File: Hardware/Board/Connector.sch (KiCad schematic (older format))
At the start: 7 parts, among them J10 WAGO_Klemmleiste_8-pol, J11 RJ12, J12 RJ45, J13 WAGO_Klemmleiste_6-pol, J7 WAGO_Klemmleiste_6-pol, J8 WAGO_Klemmleiste_4-pol, J9 WAGO_Klemmleiste_8-pol

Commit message: Eine Menge Arbeit auf der GPN, fast fertig im Schaltplan.
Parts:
- J10, J9: symbol WAGO~Klemmleisten:WAGO_Klemmleiste_8-pol -> Womo-rescue:WAGO_Klemmleiste_8-pol-WAGO_Klemmleisten
- J13, J7: symbol WAGO~Klemmleisten:WAGO_Klemmleiste_6-pol -> Womo-rescue:WAGO_Klemmleiste_6-pol-WAGO_Klemmleisten
- J8: symbol WAGO~Klemmleisten:WAGO_Klemmleiste_4-pol -> Womo-rescue:WAGO_Klemmleiste_4-pol-WAGO_Klemmleisten
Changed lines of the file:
@@
 EESchema Schematic File Version 4
 LIBS:Womo-cache
-EELAYER 26 0
+EELAYER 29 0
 EELAYER END
 $Descr A4 11693 8268
 encoding utf-8
-Sheet 7 7
+Sheet 6 7
 Title ""
 Date ""
@@
 $EndDescr
 $Comp
-L WAGO~Klemmleisten:WAGO_Klemmleiste_4-pol J8
+L Womo-rescue:WAGO_Klemmleiste_4-pol-WAGO_Klemmleisten J8
 U 1 1 5CB5F9FC
 P 1900 950
@@
 $EndComp
 $Comp
-L WAGO~Klemmleisten:WAGO_Klemmleiste_8-pol J9
+L Womo-rescue:WAGO_Klemmleiste_8-pol-WAGO_Klemmleisten J9
 U 1 1 5CB5FBA8
 P 1900 2050
@@
 $EndComp
 $Comp
-L WAGO~Klemmleisten:WAGO_Klemmleiste_8-pol J10
+L Womo-rescue:WAGO_Klemmleiste_8-pol-WAGO_Klemmleisten J10
 U 1 1 5CB5FC2E
 P 1900 3450
@@
 $EndComp
 $Comp
-L WAGO~Klemmleisten:WAGO_Klemmleiste_6-pol J7
+L Womo-rescue:WAGO_Klemmleiste_6-pol-WAGO_Klemmleisten J7
 U 1 1 5CBD1756
 P 1850 5700
@@
 	700  600  700  1450
 $Comp
-L WAGO~Klemmleisten:WAGO_Klemmleiste_6-pol J13
+L Womo-rescue:WAGO_Klemmleiste_6-pol-WAGO_Klemmleisten J13
 U 1 1 5CBE3A31
 P 5250 1050

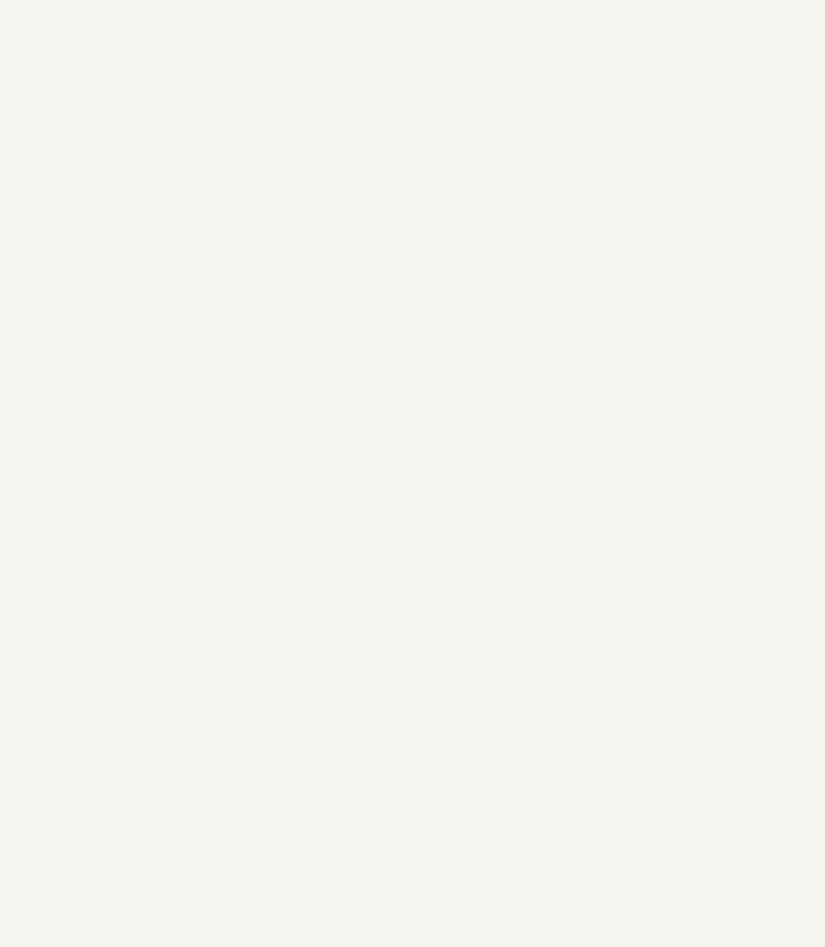
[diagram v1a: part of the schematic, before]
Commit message: Board to Board Verbindung eingefügt
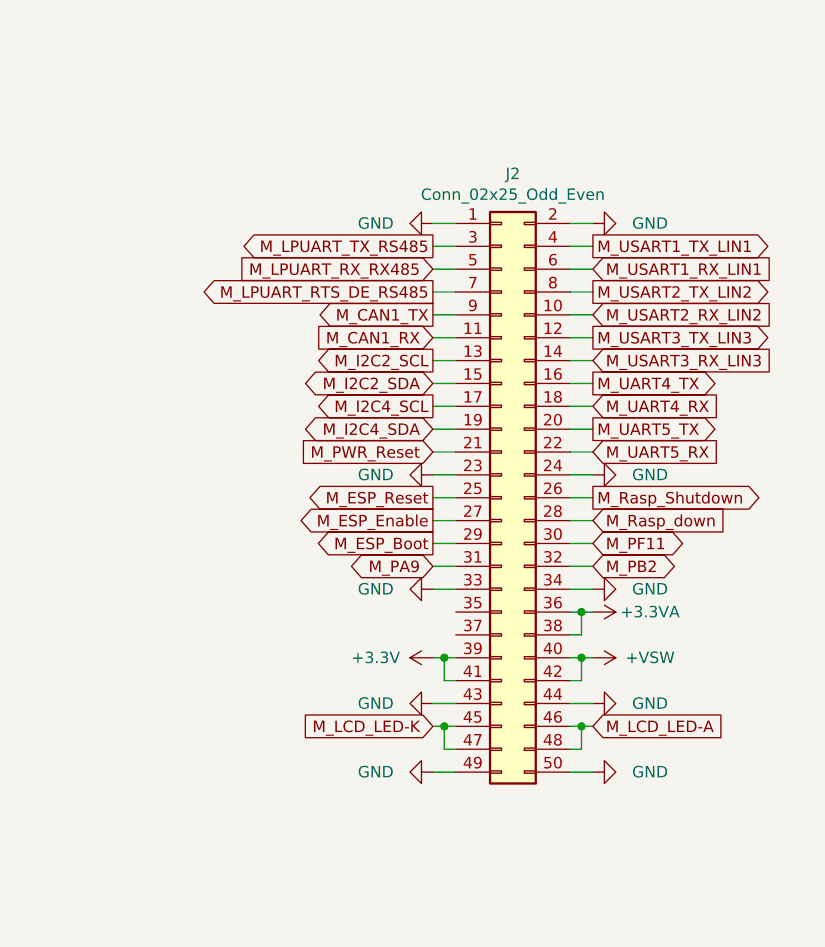
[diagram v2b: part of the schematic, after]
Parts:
- added J2: Conn_02x25_Odd_Even, Connector_PinSocket_2.54mm:PinSocket_2x25_P2.54mm_Vertical, symbol Connector_Generic:Conn_02x25_Odd_Even
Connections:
- net GND: now also J2.1 (Pin_1), J2.2 (Pin_2), J2.23 (Pin_23), J2.24 (Pin_24), J2.33 (Pin_33), J2.34 (Pin_34), J2.43 (Pin_43), J2.44 (Pin_44), J2.49 (Pin_49), J2.50 (Pin_50)
- new net +3.3VA: J2.36 (Pin_36), J2.38 (Pin_38)
- new net +3V3: J2.39 (Pin_39), J2.41 (Pin_41)
- new net +VSW: J2.40 (Pin_40), J2.42 (Pin_42)
- new net M_CAN1_RX: J2.11 (Pin_11)
- new net M_CAN1_TX: J2.9 (Pin_9)
- new net M_ESP_Boot: J2.29 (Pin_29)
- new net M_ESP_Enable: J2.27 (Pin_27)
- new net M_ESP_Reset: J2.25 (Pin_25)
- new net M_I2C2_SCL: J2.13 (Pin_13)
- new net M_I2C2_SDA: J2.15 (Pin_15)
- new net M_I2C4_SCL: J2.17 (Pin_17)
- new net M_I2C4_SDA: J2.19 (Pin_19)
- new net M_LCD_LED-A: J2.46 (Pin_46), J2.48 (Pin_48)
- new net M_LCD_LED-K: J2.45 (Pin_45), J2.47 (Pin_47)
- new net M_LPUART_RTS_DE_RS485: J2.7 (Pin_7)
- new net M_LPUART_RX_RX485: J2.5 (Pin_5)
- new net M_LPUART_TX_RS485: J2.3 (Pin_3)
- new net M_PA9: J2.31 (Pin_31)
- new net M_PB2: J2.32 (Pin_32)
- new net M_PF11: J2.30 (Pin_30)
- new net M_PWR_Reset: J2.21 (Pin_21)
- new net M_Rasp_Shutdown: J2.26 (Pin_26)
- new net M_Rasp_down: J2.28 (Pin_28)
- new net M_UART4_RX: J2.18 (Pin_18)
- new net M_UART4_TX: J2.16 (Pin_16)
- new net M_UART5_RX: J2.22 (Pin_22)
- new net M_UART5_TX: J2.20 (Pin_20)
- new net M_USART1_RX_LIN1: J2.6 (Pin_6)
- new net M_USART1_TX_LIN1: J2.4 (Pin_4)
- new net M_USART2_RX_LIN2: J2.10 (Pin_10)
- new net M_USART2_TX_LIN2: J2.8 (Pin_8)
- new net M_USART3_RX_LIN3: J2.14 (Pin_14)
- new net M_USART3_TX_LIN3: J2.12 (Pin_12)
